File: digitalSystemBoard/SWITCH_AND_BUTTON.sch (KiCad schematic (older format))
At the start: 65 parts, among them Q10 BC847, Q11 BC847, Q12 BC847, Q13 BC847, Q14 BC847, Q15 BC847, Q16 BC847, Q17 BC847, U10 IO_Switch, U11 IO_Switch, U12 IO_Switch, U13 IO_Switch, U14 74LS04, U15 Potentiometer, U6 IO_Switch, U7 IO_Switch, U8 IO_Switch, U9 IO_Switch

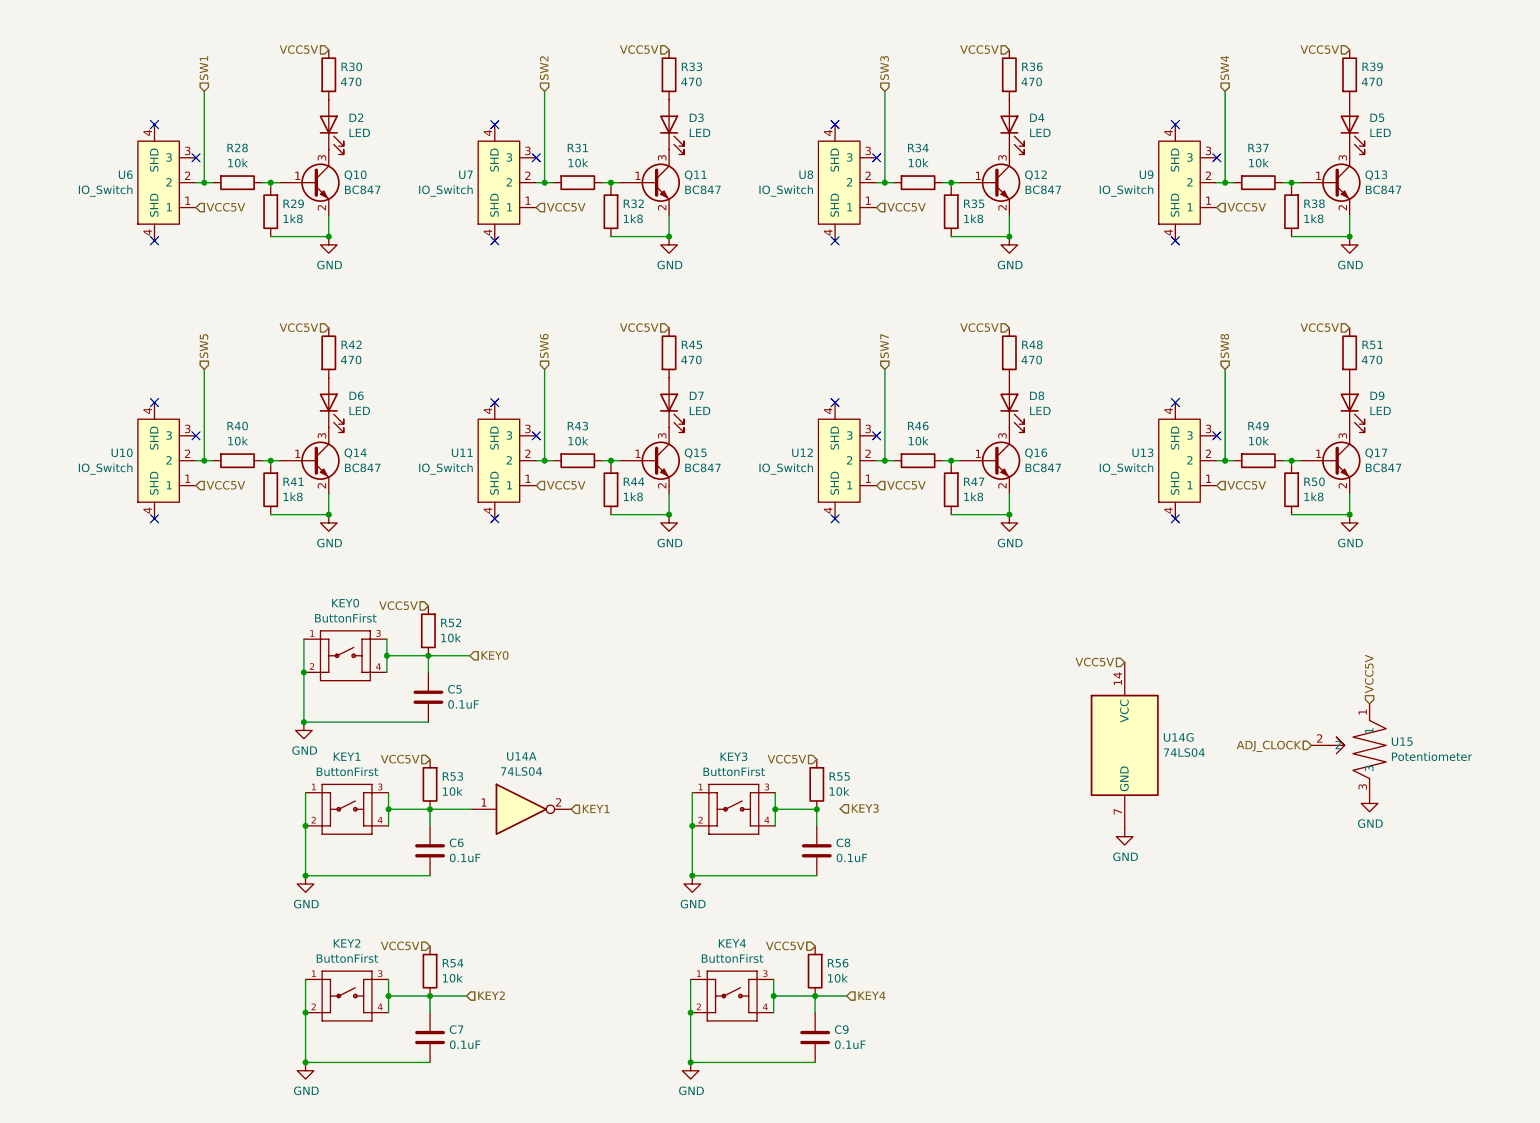
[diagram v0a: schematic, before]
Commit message: Change grid size of all schematic
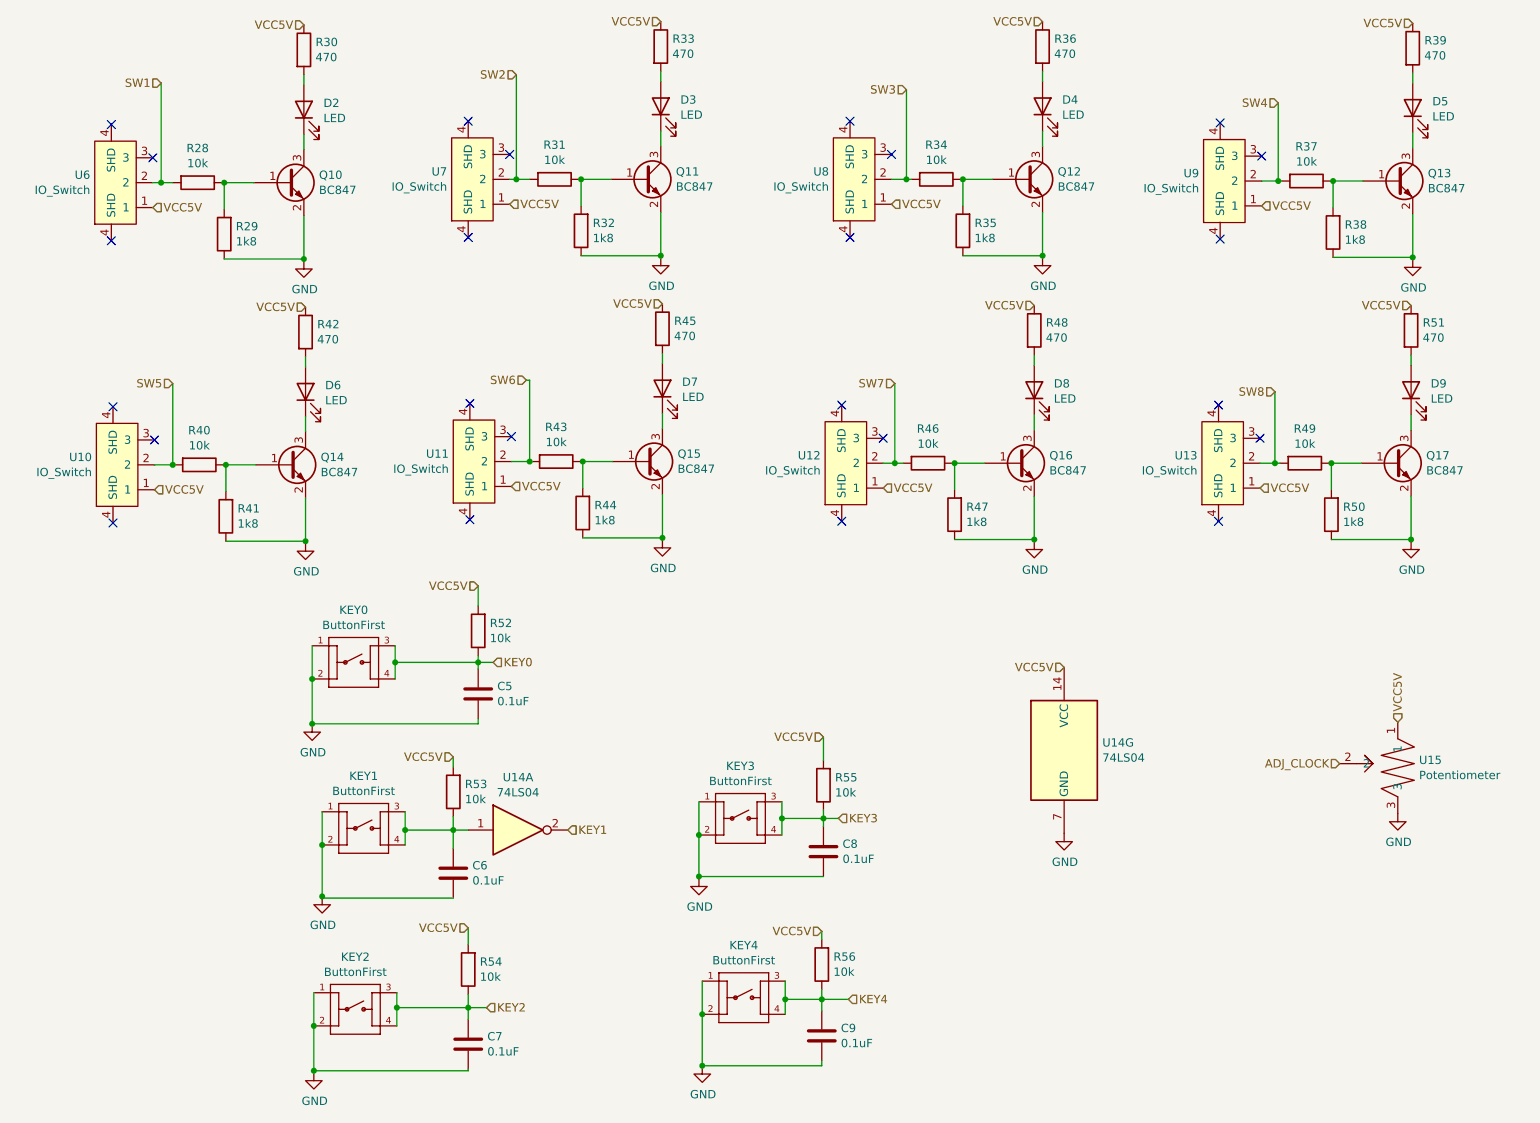
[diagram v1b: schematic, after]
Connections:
- net KEY3: now also C8.2, KEY3.3, KEY3.4, R55.1
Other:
- moved on the sheet: C5, C6, C7, C8, C9, D2, KEY0, KEY1, KEY2, KEY3, KEY4, Q10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

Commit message: Update Schematic for review
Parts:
- C5, C6, C7, C8, C9: footprint (none) -> Capacitor_SMD:C_0603_1608Metric
- D2, D3, D4, D5, D6, D7, D8, D9: footprint (none) -> LED_SMD:LED_PLCC-2
- KEY0, KEY1: footprint TE_4-1437565-9 -> digitalSystemBoard:Button
- KEY2, KEY3, KEY4: footprint TE_4-1437565-9 -> digitalSystemBoard:Button_CLOCK
- R28, R29, R30, R31, R32, R33, R34, R35, R36, R37, R38, R39, R40, R41, R42, R43, R44, R45, R46, R47, R48, R49, R50, R51, R52, R53, R54, R55, R56: footprint (none) -> Resistor_SMD:R_0603_1608Metric
- U10, U11, U12, U13, U6, U7, U8, U9: footprint (none) -> digitalSystemBoard:SS-12F44G5
- U15: footprint (none) -> digitalSystemBoard:RV09S
